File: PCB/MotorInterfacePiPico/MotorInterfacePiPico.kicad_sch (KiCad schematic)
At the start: 29 parts, among them J1 Motor Connector, J2 Screw_Terminal_01x06, Q1 2N3904, Q2 2N3904, Q3 2N3904, U1 Pico, U2 OPA4197

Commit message: Layout complete, need BOM
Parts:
- U2: footprint Package_SO:SOIC-14_3.9x8.7mm_P1.27mm -> TJR:D14_TEX
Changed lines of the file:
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@@
 			)
 		)
-		(property "Footprint" "Package_SO:SOIC-14_3.9x8.7mm_P1.27mm"
+		(property "Footprint" "TJR:D14_TEX"
 			(at 209.55 91.44 0)
 			(effects
@@
 			)
 		)
-		(property "Footprint" "Package_SO:SOIC-14_3.9x8.7mm_P1.27mm"
+		(property "Footprint" "TJR:D14_TEX"
 			(at 209.55 26.67 0)
 			(effects
@@
 			)
 		)
-		(property "Footprint" "Package_SO:SOIC-14_3.9x8.7mm_P1.27mm"
+		(property "Footprint" "TJR:D14_TEX"
 			(at 209.55 58.42 0)
 			(effects

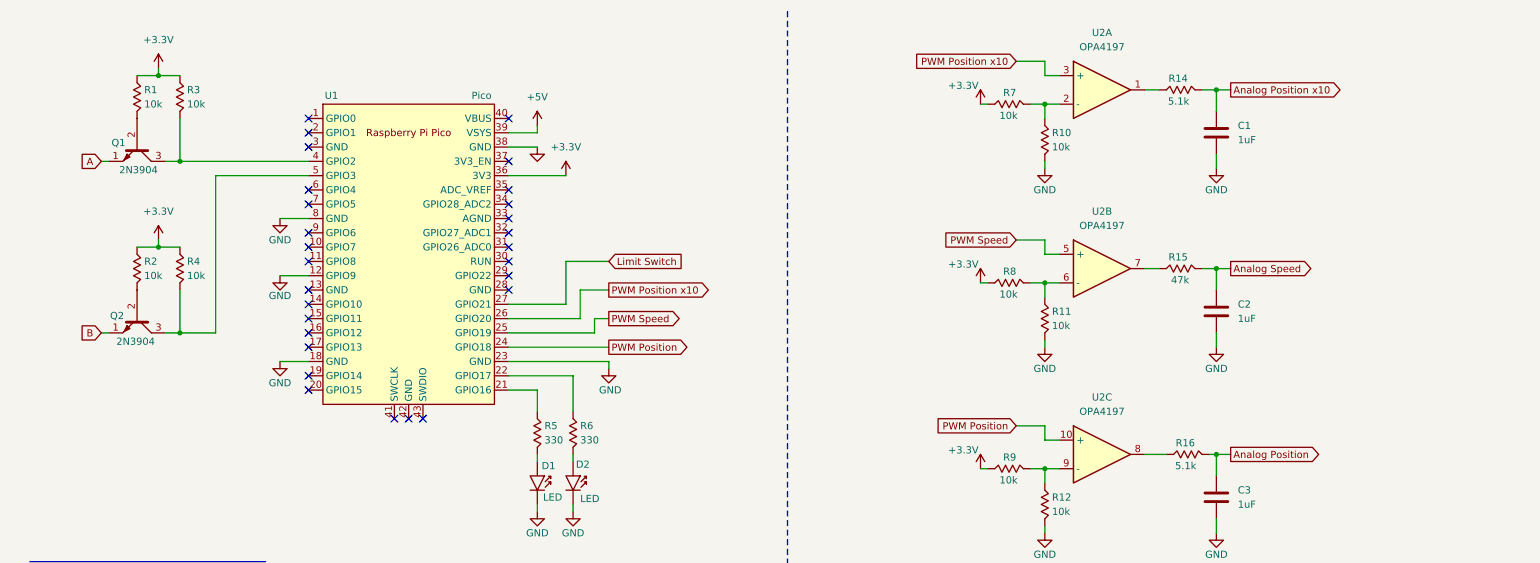
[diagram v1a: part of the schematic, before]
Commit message: add MotorInterfacePiPico
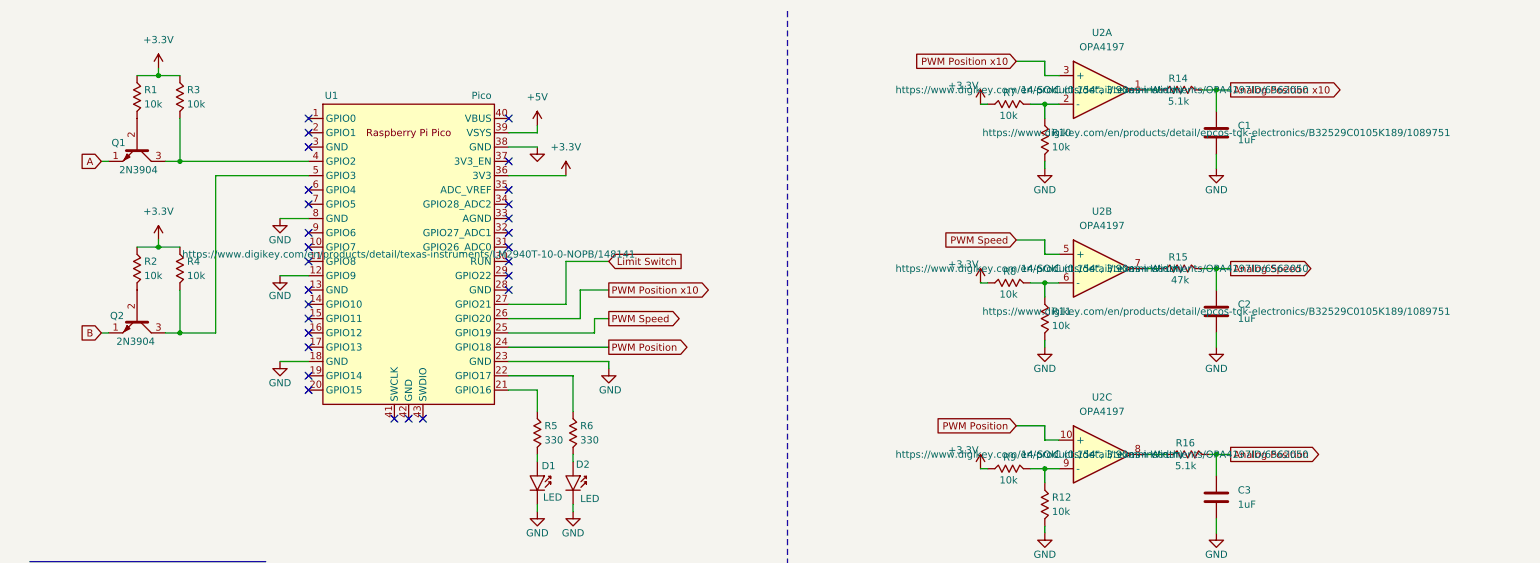
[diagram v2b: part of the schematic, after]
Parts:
- C1, C2: digikey (none) -> https://www.digikey.com/en/products/detail/epcos-tdk-electr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
- U1: digikey (none) -> https://www.digikey.com/en/products/detail/texas-instrument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
- U2: Notes (none) -> 14-SOIC (0.154", 3.90mm Width); digikey (none) -> https://www.digikey.com/en/products/detail/texas-instrument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
